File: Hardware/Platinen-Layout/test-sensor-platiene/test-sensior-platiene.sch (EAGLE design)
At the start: 38 parts, among them J10 Flash Programming, J5 Flash Programming, U1 AS72651, U10 4MB Flash, U2 4MB Flash, U5 AS72653, U6 AS72652, U9 IR

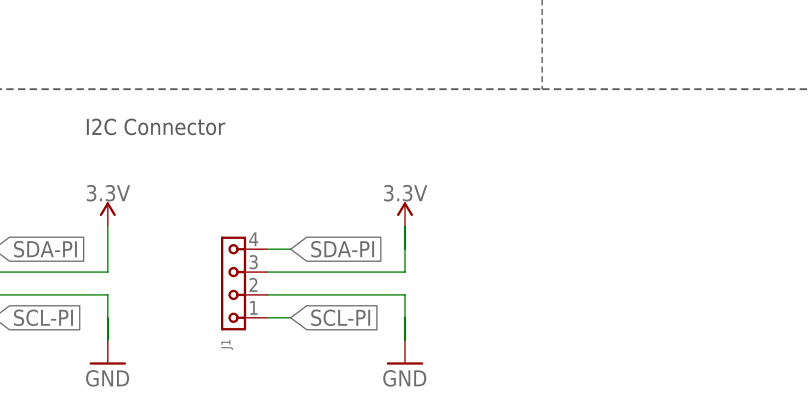
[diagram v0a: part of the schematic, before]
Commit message: board is better
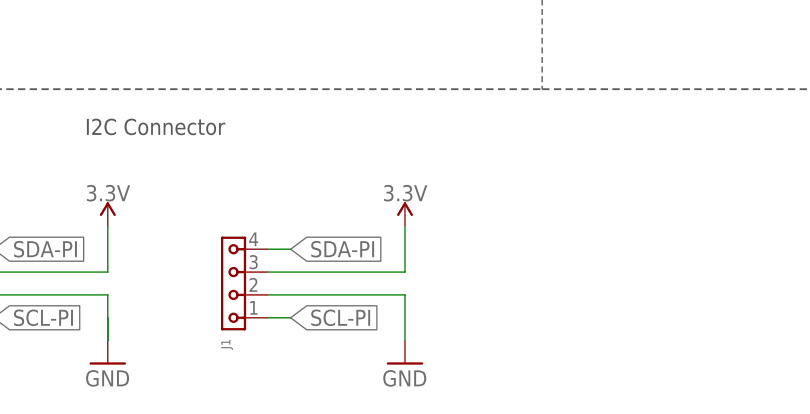
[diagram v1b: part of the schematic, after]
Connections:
- removed net N$10: J1.3
- removed net N$8: J1.2
- net 3.3V: now also J1.3
- net GND: now also J1.2
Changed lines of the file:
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@@
 <junction x="271.78" y="187.96"/>
+</segment>
+<segment>
+<pinref part="J1" gate="G$1" pin="2"/>
+<wire x1="170.18" y1="38.1" x2="185.42" y2="38.1" width="0.1524" layer="91"/>
+<wire x1="185.42" y1="38.1" x2="185.42" y2="33.02" width="0.1524" layer="91"/>
+<pinref part="GND3" gate="1" pin="GND"/>
 </segment>
 </net>
@@
 <wire x1="152.4" y1="40.64" x2="152.4" y2="45.72" width="0.1524" layer="91"/>
 </segment>
+<segment>
+<pinref part="J1" gate="G$1" pin="3"/>
+<pinref part="SUPPLY3" gate="G$1" pin="3.3V"/>
+<wire x1="185.42" y1="45.72" x2="185.42" y2="40.64" width="0.1524" layer="91"/>
+<wire x1="170.18" y1="40.64" x2="185.42" y2="40.64" width="0.1524" layer="91"/>
+</segment>
 </net>
 <net name="I2C_ENB" class="0">
@@
 </segment>
 </net>
-<net name="N$8" class="0">
-<segment>
-<wire x1="185.42" y1="33.02" x2="185.42" y2="35.56" width="0.1524" layer="91"/>
-<pinref part="J1" gate="G$1" pin="2"/>
-<wire x1="170.18" y1="38.1" x2="185.42" y2="38.1" width="0.1524" layer="91"/>
-<wire x1="185.42" y1="38.1" x2="185.42" y2="33.02" width="0.1524" layer="91"/>
-<pinref part="GND3" gate="1" pin="GND"/>
-</segment>
-</net>
-<net name="N$10" class="1">
-<segment>
-<wire x1="185.42" y1="45.72" x2="185.42" y2="43.18" width="0.1524" layer="91"/>
-<pinref part="J1" gate="G$1" pin="3"/>
-<wire x1="170.18" y1="40.64" x2="185.42" y2="40.64" width="0.1524" layer="91"/>
-<wire x1="185.42" y1="40.64" x2="185.42" y2="45.72" width="0.1524" layer="91"/>
-<pinref part="SUPPLY3" gate="G$1" pin="3.3V"/>
-</segment>
-</net>

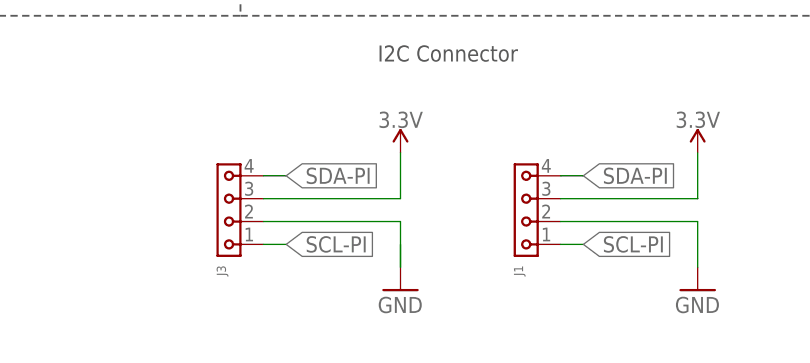
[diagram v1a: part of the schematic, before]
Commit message: board is better2
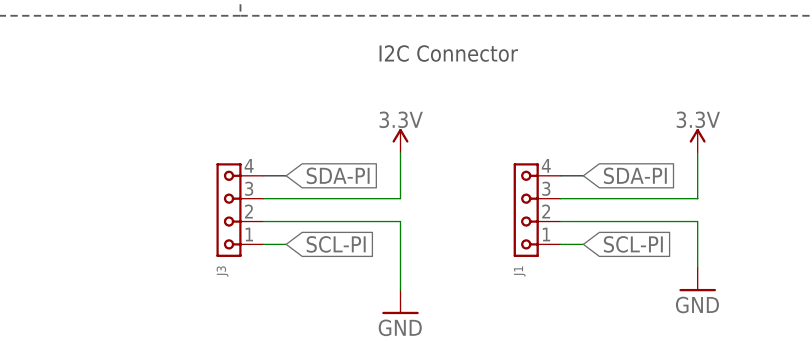
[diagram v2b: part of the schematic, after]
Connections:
- removed net N$11: J3.2
- net GND: now also J3.2
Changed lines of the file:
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@@
 <attribute name="VALUE" x="167.68" y="33.27" size="1.016" layer="96" rot="R90" align="bottom-right"/>
 </instance>
-<instance part="GND19" gate="1" x="152.4" y="30.48" smashed="yes">
-<attribute name="VALUE" x="149.86" y="27.94" size="1.778" layer="96"/>
+<instance part="GND19" gate="1" x="152.4" y="27.94" smashed="yes">
+<attribute name="VALUE" x="149.86" y="25.4" size="1.778" layer="96"/>
 </instance>
 <instance part="GND3" gate="1" x="185.42" y="30.48" smashed="yes">
@@
 <pinref part="GND3" gate="1" pin="GND"/>
 </segment>
+<segment>
+<pinref part="J3" gate="G$1" pin="2"/>
+<wire x1="137.16" y1="38.1" x2="152.4" y2="38.1" width="0.1524" layer="91"/>
+<pinref part="GND19" gate="1" pin="GND"/>
+<wire x1="152.4" y1="38.1" x2="152.4" y2="30.48" width="0.1524" layer="91"/>
+</segment>
 </net>
 <net name="SCL-PI" class="0">
@@
 </segment>
 </net>
-<net name="N$11" class="0">
-<segment>
-<wire x1="152.4" y1="33.02" x2="152.4" y2="35.56" width="0.1524" layer="91"/>
-<pinref part="J3" gate="G$1" pin="2"/>
-<wire x1="137.16" y1="38.1" x2="152.4" y2="38.1" width="0.1524" layer="91"/>
-<wire x1="152.4" y1="38.1" x2="152.4" y2="33.02" width="0.1524" layer="91"/>
-<pinref part="GND19" gate="1" pin="GND"/>
-</segment>
-</net>
